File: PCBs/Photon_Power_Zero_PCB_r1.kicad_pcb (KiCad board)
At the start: 2 copper layers, 30.1 x 65.1 mm, 56 parts, among them J1 JST_S2B-PH-SM4-TB_LF__SN_, J2 JST_GH_SM02B-GHS-TB_1x02-1MP_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, J3 SMT_Solar_barrel, U1 ATtiny84-SSFR, U2 REG_MCP1700T-3602E/MB, U3 bq2407, U4 AP2161-WG, U5 TPS613222A

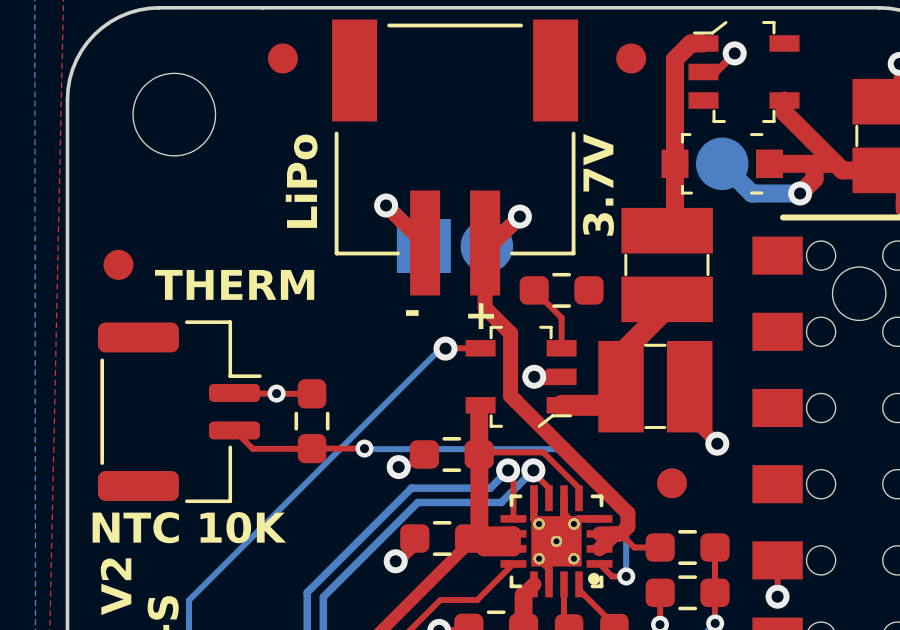
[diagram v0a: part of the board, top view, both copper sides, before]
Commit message: minor pcb and schematic updates!
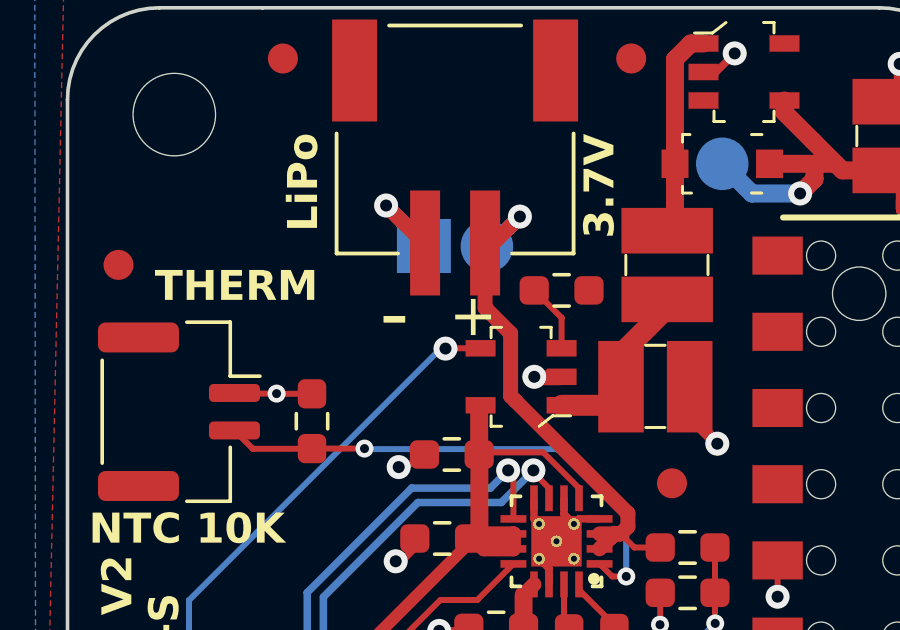
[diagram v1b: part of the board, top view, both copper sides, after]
